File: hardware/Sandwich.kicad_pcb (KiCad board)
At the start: 2 copper layers, 80 x 100.2 mm, 20 parts, among them P1 CONN_01X20, P2 CONN_01X06, P3 VGA_OUT, Q1 PZT2222A, U1 P8X32A-D40, U2 24C512, Y1 5MHz

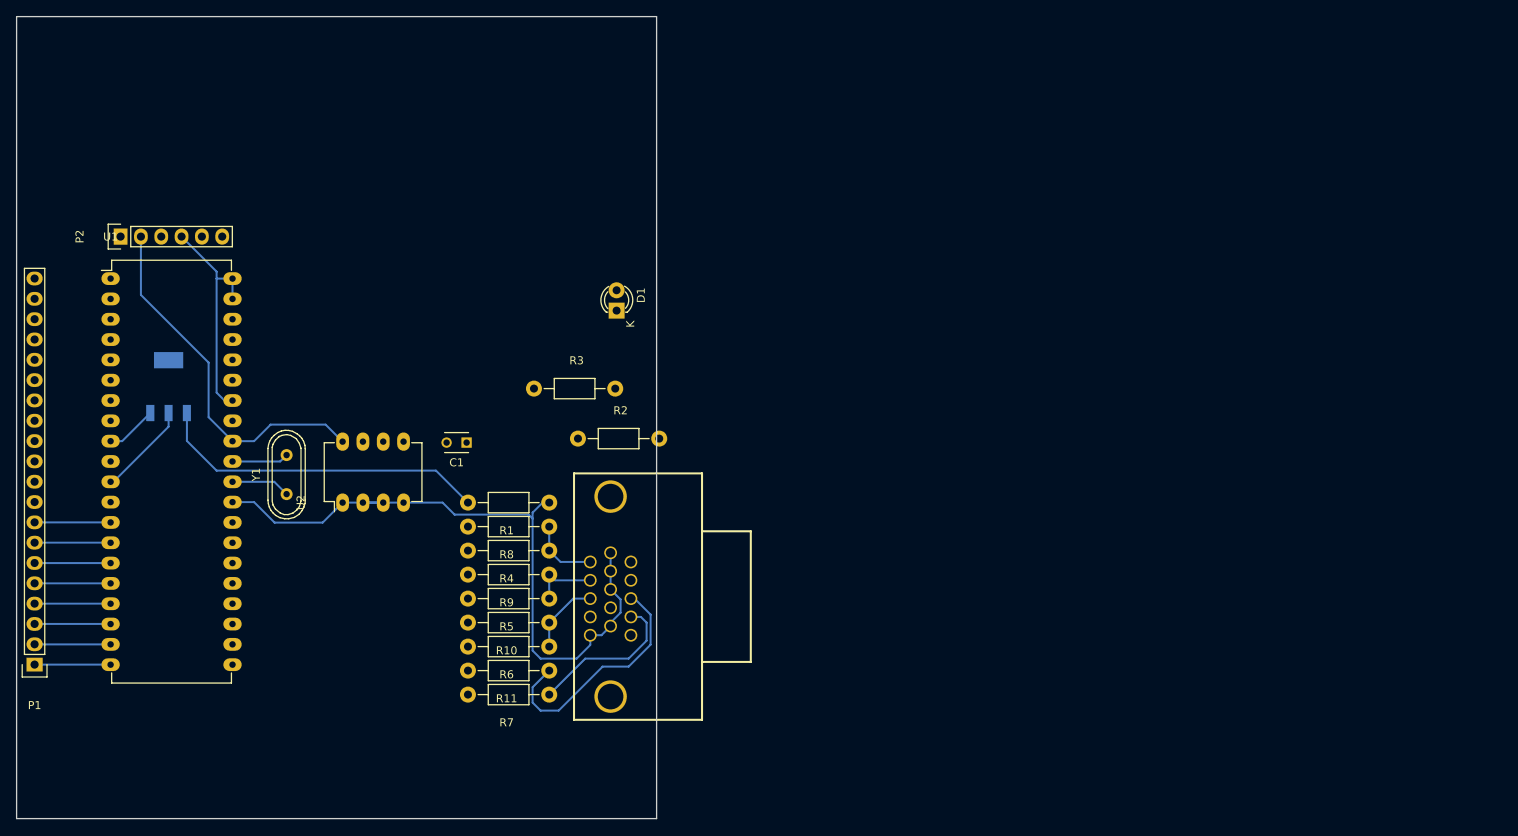
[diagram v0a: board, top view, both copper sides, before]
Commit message: Updated schematics, PCB layout is nearly done.
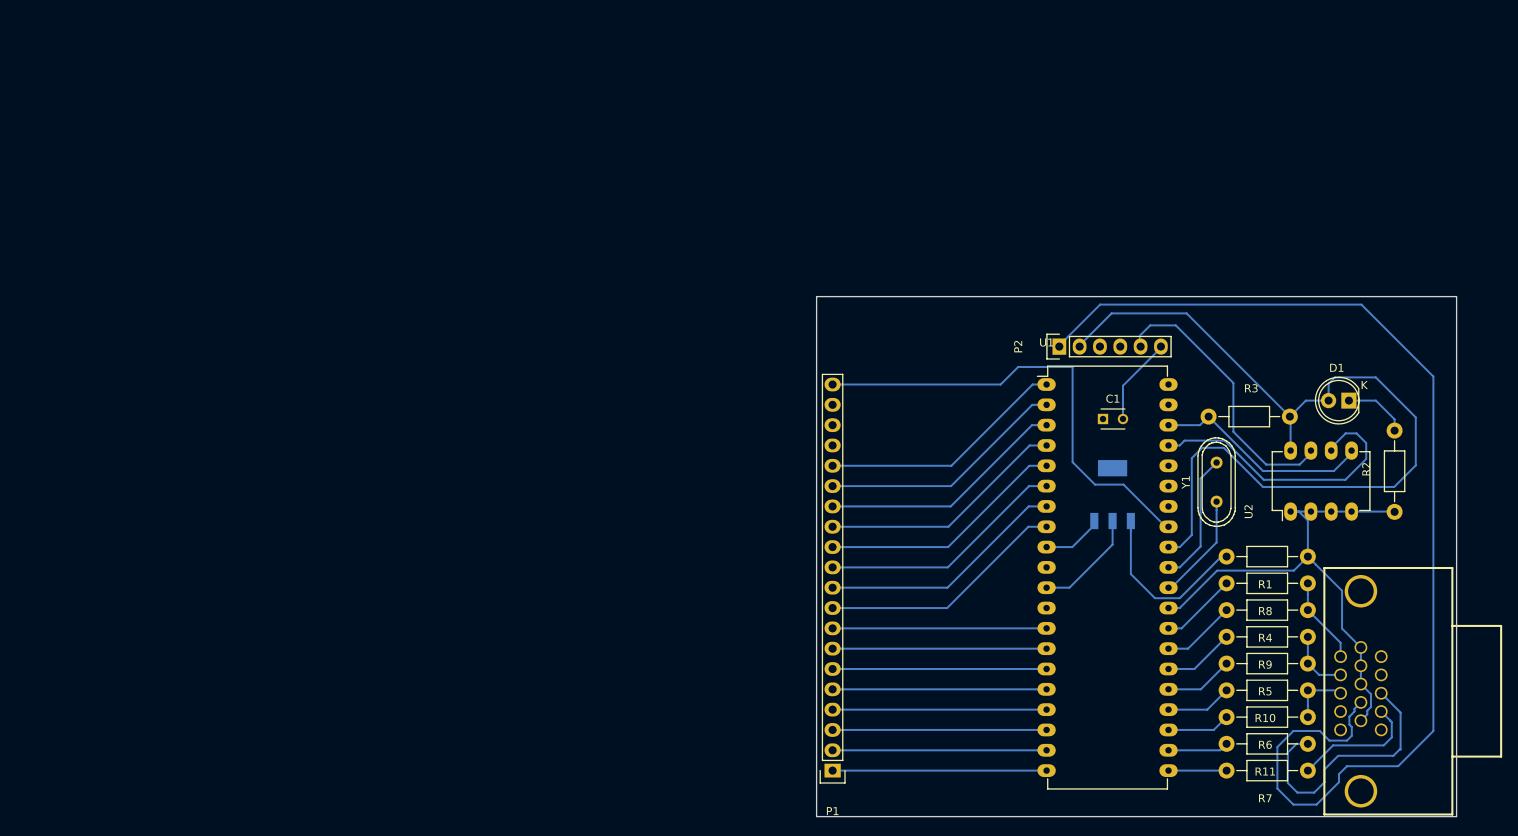
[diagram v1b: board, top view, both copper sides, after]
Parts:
- D1: footprint LEDs:LED-3MM -> LEDs:LED-5MM
- moved Q1 118.8 mm to (187.0, 109.8)
- moved U2 118.5 mm to (209.2, 111.9)
- moved P2 118.1 mm to (180.3, 91.2)
- moved U1 117.7 mm to (178.8, 96.0)
- moved Y1 116.3 mm to (200.0, 108.2)
- moved P1 100.6 mm to (152.0, 144.2)
- moved R7 100.4 mm to (211.4, 144.2)
- moved R11 100.3 mm to (211.4, 140.9)
- moved R6 100.3 mm to (211.4, 137.6)
- moved R10 100.3 mm to (211.4, 134.2)
- moved R5 100.2 mm to (211.4, 130.9)
- moved R9 100.2 mm to (211.4, 127.5)
- moved R4 100.2 mm to (211.4, 124.2)
- moved R8 100.2 mm to (211.4, 120.8)
- moved R1 100.1 mm to (211.4, 117.5)
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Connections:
- P2 pad 5: PROP_DTR -> GND
- P2 pad 6: GND -> PROP_DTR
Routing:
- net 5V: track 0.00 -> 142.7 mm
- net 3.3V: track 45.8 -> 110.0 mm
- net Net-(P1-Pad20): track 0.00 -> 58.1 mm
- net Net-(U1-Pad37): track 0.00 -> 36.0 mm
- net Net-(P1-Pad9): track 0.00 -> 31.0 mm
- net Net-(P1-Pad16): track 0.00 -> 31.0 mm
- net Net-(P1-Pad14): track 0.00 -> 31.0 mm
- net Net-(P1-Pad15): track 0.00 -> 31.0 mm
- net Net-(P1-Pad13): track 0.00 -> 31.0 mm
- net Net-(P1-Pad12): track 0.00 -> 31.0 mm
- net Net-(P1-Pad11): track 0.00 -> 31.0 mm
- net Net-(P1-Pad10): track 0.00 -> 31.0 mm
- net PROP_RX: track 28.2 -> 0.00 mm
- net Net-(R3-Pad1): track 0.00 -> 27.4 mm
- net Net-(C1-Pad1): track 41.8 -> 22.0 mm
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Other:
- board size 80 x 100.2 mm -> 80 x 65 mm
